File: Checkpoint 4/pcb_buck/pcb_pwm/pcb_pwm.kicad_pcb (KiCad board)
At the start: 2 copper layers, 55.7 x 39.2 mm, 15 parts, among them J1 Conn_01x04_Socket, J2 Conn_01x03_Socket, U1 TL082, U3 LM393

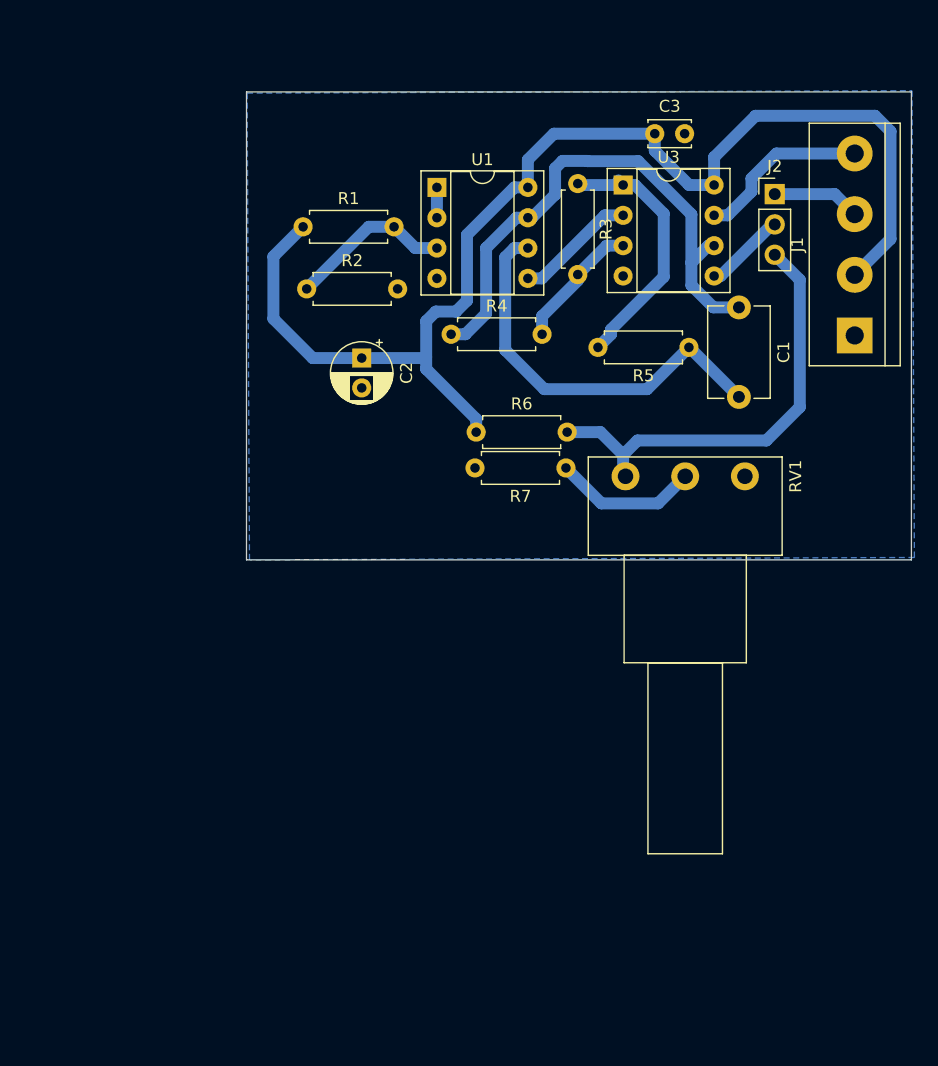
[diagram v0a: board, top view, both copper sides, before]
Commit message: pcb pwm
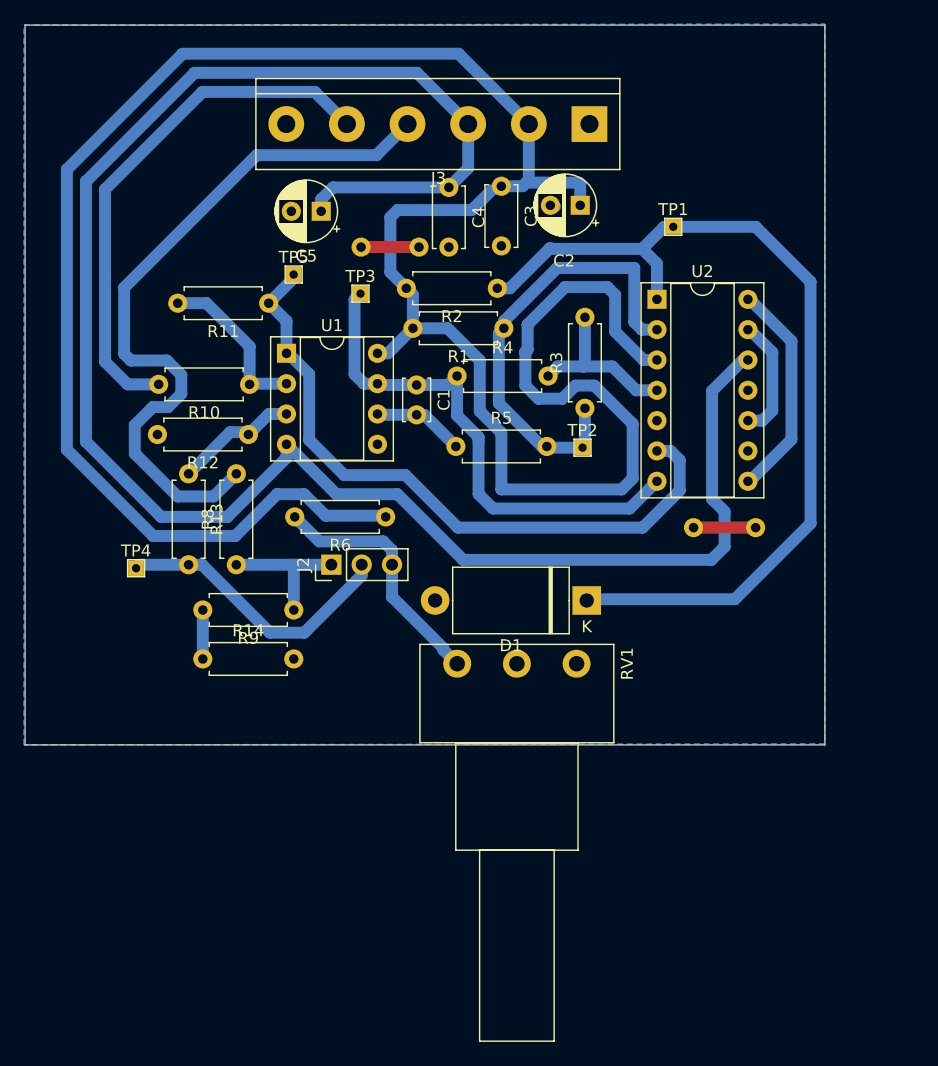
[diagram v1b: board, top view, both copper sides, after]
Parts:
- removed J1: Conn_01x04_Socket, TerminalBlock:TerminalBlock_bornier-4_P5.08mm
- removed R7: 2,7k, Resistor_THT:R_Axial_DIN0207_L6.3mm_D2.5mm_P7.62mm_Horizontal
- removed U3: LM393, Package_DIP:DIP-8_W7.62mm_Socket
- added ?: , , F.Cu at (144.0, 77.7)
- added ?: , , F.Cu at (167.0, 101.2)
- added ?: , , F.Cu at (172.2, 101.2)
- added ?: , , F.Cu at (139.2, 77.7)
- added C4: 10n, Capacitor_THT:C_Disc_D5.0mm_W2.5mm_P5.00mm, F.Cu at (146.5, 72.7)
- added C5: 10u, Capacitor_THT:CP_Radial_D5.0mm_P2.50mm, F.Cu at (135.8, 74.7)
- added D1: D_Schottky, Diode_THT:D_DO-27_P12.70mm_Horizontal, F.Cu at (158.1, 107.3)
- added J3: Conn_01x06_Socket, TerminalBlock:TerminalBlock_bornier-6_P5.08mm, F.Cu at (158.3, 67.4)
- added R10: 100k, Resistor_THT:R_Axial_DIN0207_L6.3mm_D2.5mm_P7.62mm_Horizontal, F.Cu at (129.8, 89.2)
- added R11: 100k, Resistor_THT:R_Axial_DIN0207_L6.3mm_D2.5mm_P7.62mm_Horizontal, F.Cu at (131.4, 82.4)
- added R12: 100k, Resistor_THT:R_Axial_DIN0207_L6.3mm_D2.5mm_P7.62mm_Horizontal, F.Cu at (129.7, 93.4)
- added R13: 100k, Resistor_THT:R_Axial_DIN0207_L6.3mm_D2.5mm_P7.62mm_Horizontal, F.Cu at (124.7, 96.7)
- added R14: 10, Resistor_THT:R_Axial_DIN0207_L6.3mm_D2.5mm_P7.62mm_Horizontal, F.Cu at (125.9, 112.2)
- added R8: 120, Resistor_THT:R_Axial_DIN0207_L6.3mm_D2.5mm_P7.62mm_Horizontal, F.Cu at (128.7, 104.3)
- added R9: 68, Resistor_THT:R_Axial_DIN0207_L6.3mm_D2.5mm_P7.62mm_Horizontal, F.Cu at (133.5, 108.1)
- added TP1: Vo, TestPoint:TestPoint_THTPad_1.3x1.3mm_Drill0.7mm, F.Cu at (165.3, 76.0)
- added TP2: Vcuad, TestPoint:TestPoint_THTPad_1.3x1.3mm_Drill0.7mm, F.Cu at (157.7, 94.5)
- added TP3: Vtriang, TestPoint:TestPoint_THTPad_1.3x1.3mm_Drill0.7mm, F.Cu at (139.1, 81.6)
- added TP4: Vcomp, TestPoint:TestPoint_THTPad_1.3x1.3mm_Drill0.7mm, F.Cu at (120.3, 104.6)
- added TP5: Verr, TestPoint:TestPoint_THTPad_1.3x1.3mm_Drill0.7mm, F.Cu at (133.5, 80.0)
- added U2: LM2901, Package_DIP:DIP-14_W7.62mm_Socket, F.Cu at (163.9, 82.1)
- C1: footprint Capacitor_THT:C_Disc_D7.5mm_W5.0mm_P7.50mm -> Capacitor_THT:C_Disc_D3.4mm_W2.1mm_P2.50mm
- C3: footprint Capacitor_THT:C_Disc_D3.4mm_W2.1mm_P2.50mm -> Capacitor_THT:C_Disc_D5.0mm_W2.5mm_P5.00mm
- R1: value 89k -> 10k
- R2: value 100k -> 10k
- R3: value 100k -> 220k
- R4: value 27k -> 5,1k
- R5: value 33k -> 39k
- R6: value 5,1k -> 8,2k
- moved J2 48.4 mm to (136.7, 104.3), turned to 90 degrees
- moved C1 27.8 mm to (143.8, 89.2)
- moved C2 22.3 mm to (157.5, 74.2), turned to 180 degrees
- moved R5 21.2 mm to (147.1, 94.4), turned to 0 degrees
- moved RV1 21.1 mm to (147.2, 112.6)
- moved R1 18.8 mm to (151.1, 84.5), turned to 180 degrees
- moved R3 18.8 mm to (157.9, 91.2), turned to 90 degrees
- moved U1 18.8 mm to (132.9, 86.6)
- moved R2 16.0 mm to (150.6, 81.2), turned to 180 degrees
- moved C3 13.6 mm to (150.9, 72.6), turned to -90 degrees
- moved R6 10.4 mm to (141.2, 100.3), turned to 180 degrees
- moved R4 3.54 mm to (147.2, 88.5)
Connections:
- net Net-(U3B--) renamed Vtriang
- J2 pad 1: Vsin -> Net-(J2-Pin_1)
- J2 pad 2: Net-(J2-Pin_2) -> Vcomp
- R1 pad 1: Vcc -> Vcuad
- R1 pad 2: Net-(U1A-+) -> Vcc
- R2 pad 1: Net-(U1A-+) -> Vo
- R2 pad 2: 0 -> Vcc
- R3 pad 1: Net-(R3-Pad1) -> Vcuad
- R5 pad 2: Net-(R3-Pad1) -> Vcuad
- RV1 pad 2: Net-(R7-Pad1) -> 0
- U1 pad 1: Net-(U1A--) -> Verr
- U1 pad 4: 0 -> -Vcc
- U1 pad 5: Net-(U1A--) -> 0
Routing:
- net -Vcc: track 0.00 -> 158.8 mm
- net Vcc: track 104.1 -> 204.6 mm
- net Vo: track 14.6 -> 76.7 mm
- net Verr: track 0.00 -> 56.3 mm
- net Vsin: track 7.40 -> 60.2 mm
- net Vref: track 0.00 -> 44.5 mm
- net Vcuad: track 0.00 -> 38.4 mm
- net Net-(U1B--): track 34.1 -> 7.70 mm
- net Vcomp: track 0.00 -> 24.3 mm
- net Net-(R3-Pad1): track 22.3 -> 0.00 mm
- net Net-(U2D--): track 0.00 -> 18.4 mm
- net Net-(J2-Pin_3): track 37.4 -> 21.1 mm
- net Net-(R7-Pad1): track 12.2 -> 0.00 mm
- net Net-(J2-Pin_1): track 0.00 -> 11.8 mm
- net Net-(U2C--): track 0.00 -> 10.1 mm
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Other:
- board size 55.7 x 39.2 mm -> 67 x 60.3 mm
